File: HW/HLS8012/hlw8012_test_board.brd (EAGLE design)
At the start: 29.5 x 72.4 mm, 30 parts

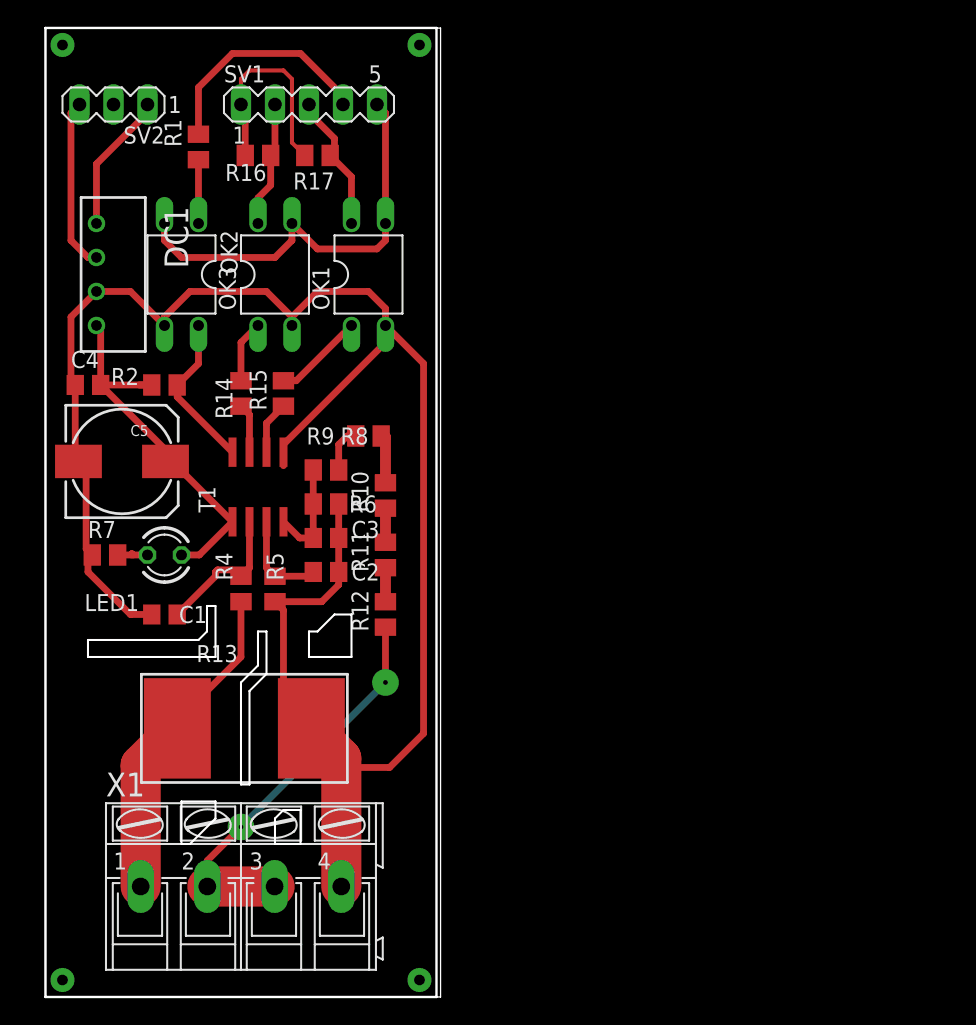
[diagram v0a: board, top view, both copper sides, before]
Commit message: Updated hlw board. Added libs
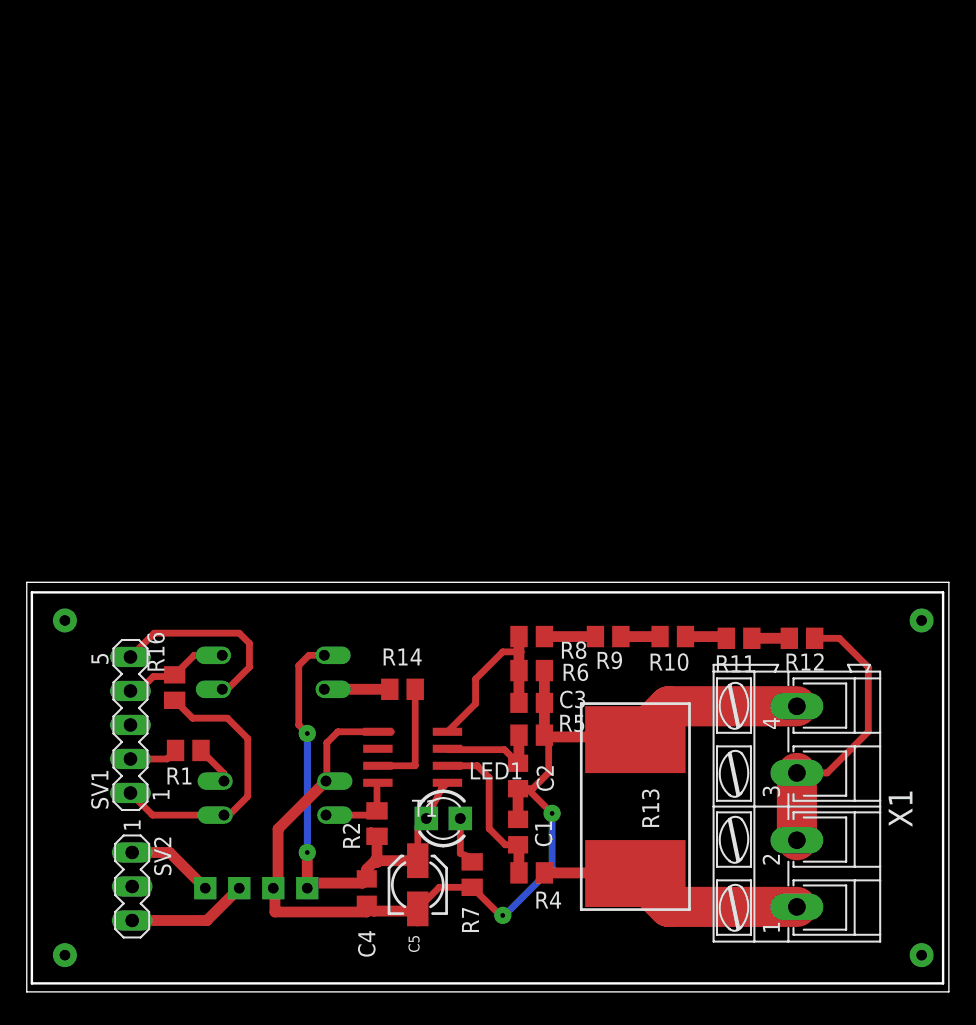
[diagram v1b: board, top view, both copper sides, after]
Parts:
- removed OK1: PC817, optocoupler:DIL04
- removed R15: 0.5K, rcl:M0805
- removed R17: 10K, rcl:M0805
- C5: value 100nF -> 10uF; device rcl:153CLV-0810 -> rcl:153CLV-0405
- DC1: value VA-1205S -> VA-0505S1
- R16: value 10K -> 2K
- R2: value 10K -> 5K
- moved SV2 58.4 mm to (8.38, 8.89), turned to 270 degrees
- moved SV1 48.2 mm to (8.26, 21.0), turned to 90 degrees
- moved DC1 47.4 mm to (17.7, 8.76), flipped to the bottom, turned to 180 degrees
- moved R1 45.1 mm to (12.6, 19.1), turned to 180 degrees
- moved C4 43.2 mm to (25.9, 8.51), turned to 90 degrees
- moved X1 42.0 mm to (58.0, 14.9), turned to 90 degrees
- moved R16 40.2 mm to (11.6, 23.7), turned to 270 degrees
- moved OK2 39.7 mm to (19.1, 15.5), flipped to the bottom, turned to 90 degrees
- moved C5 38.6 mm to (29.7, 9.02), turned to 90 degrees
- moved R2 36.4 mm to (26.7, 13.6), turned to 270 degrees
- moved R7 36.4 mm to (33.8, 9.78), turned to 90 degrees
- moved R12 31.2 mm to (58.4, 27.4), turned to 180 degrees
- moved C1 31.0 mm to (37.2, 13.0), turned to 90 degrees
- moved R4 30.4 mm to (38.2, 9.91), turned to 180 degrees
- moved R13 29.9 mm to (45.7, 14.6), turned to 90 degrees
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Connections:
- removed net N$10: R15.1, T1.6
- removed net N$12: OK1.4, R17.1, SV1.3
- removed net N$8: OK3.1, R14.2
- net GND: no longer OK1.2, OK3.2
- net N$1: now also OK2.1; no longer R17.2
- net N$16: no longer OK1.3, OK2.2
- net N$2: now also OK2.2, R1.1; no longer R1.2, SV1.4
- net N$3: now also R1.2, SV1.2; no longer OK2.1, R1.1
- net N$6: now also SV1.4; no longer SV1.2
- net N$7: now also OK3.2, R14.2; no longer OK1.1, R15.2
- net VDD: now also OK3.1
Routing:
- net GND: track 141.6 -> 88.8 mm, vias 0 -> 2
- net N$16: track 31.6 -> 14.4 mm
- net N$2: track 17.3 -> 3.00 mm
- net N$12: track 11.1 -> 0.00 mm
- net VDD: track 29.0 -> 37.9 mm, vias 0 -> 2
- net N$30: track 29.9 -> 22.5 mm, vias 2 -> 0
- net N$21: track 7.81 -> 13.8 mm
- net N$4: track 12.3 -> 6.53 mm
- net N$5: track 3.70 -> 8.50 mm
- net N$8: track 4.66 -> 0.00 mm
- net N$10: track 3.96 -> 0.00 mm
- net N$14: track 10.5 -> 6.57 mm
- net N$15: track 12.9 -> 9.00 mm
- net N$1: track 17.2 -> 21.0 mm
- net N$17: track 22.5 -> 19.9 mm
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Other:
- board size 29.5 x 72.4 mm -> 68.9 x 30.6 mm
